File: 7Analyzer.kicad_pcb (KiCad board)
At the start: 2 copper layers, 51.3 x 72.1 mm, 30 parts, among them J1 PINHD_1x1_Male, J10 PINHD_1x3_Male, J11 PINHD_1x3_Male, J2 PINHD_1x1_Male, J3 PINHD_1x3_Male, J4 PINHD_1x3_Male, J5 PINHD_1x3_Male, J6 PINHD_1x3_Male, J7 PINHD_1x3_Male, J8 PINHD_1x3_Male, J9 PINHD_1x3_Male, P1 USB_C_Plug, U1 ESP32-DevKitC

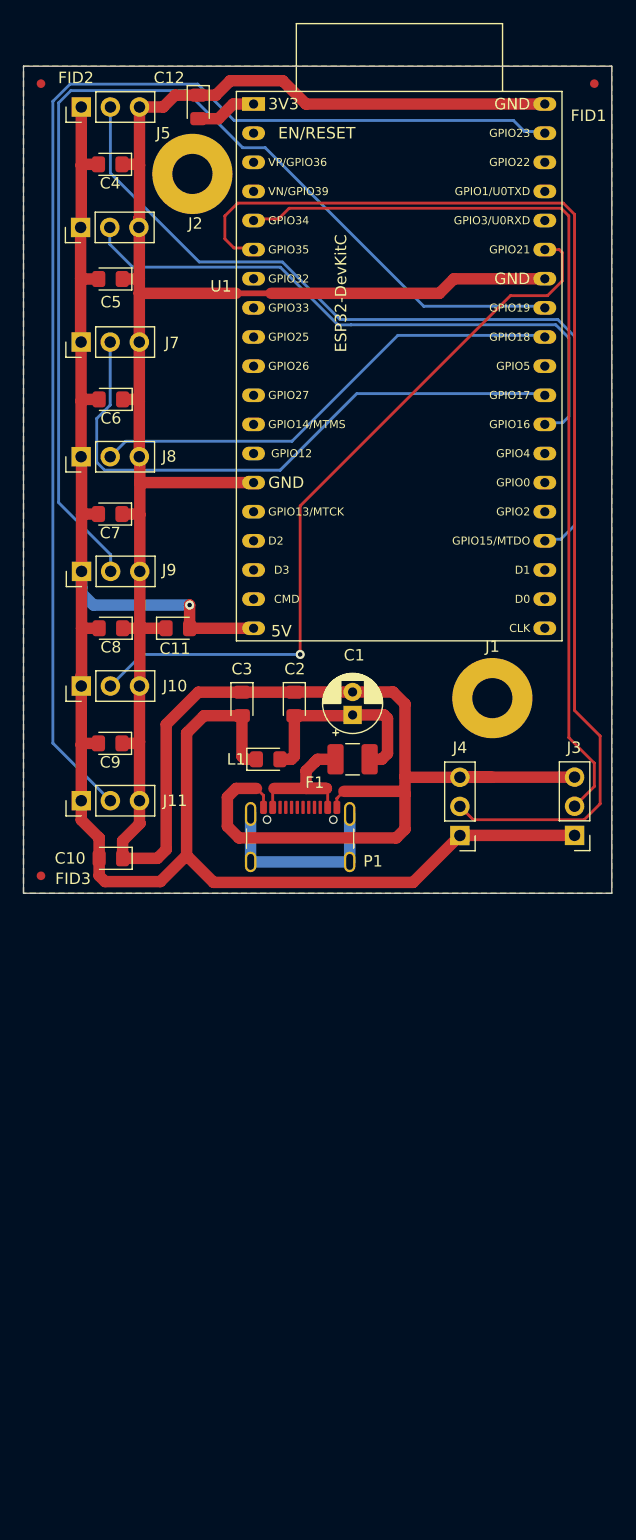
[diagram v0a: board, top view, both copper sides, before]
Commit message: laengere Version
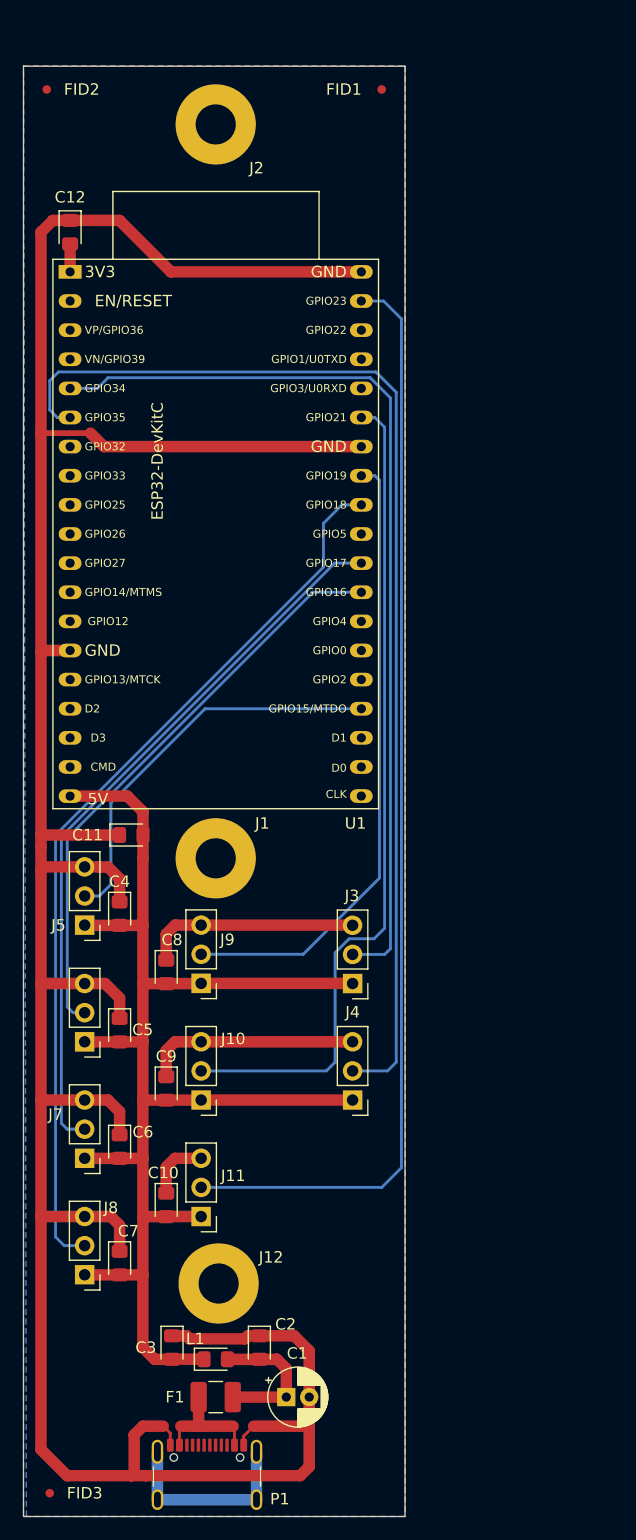
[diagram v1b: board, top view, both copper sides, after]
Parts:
- added J12: PINHD_1x1_Male, MountingHole:MountingHole_3.5mm_Pad, F.Cu at (29.0, 118.1)
- moved J5 71.4 mm to (17.3, 86.9), turned to 180 degrees
- moved J8 71.3 mm to (17.3, 117.3), turned to 180 degrees
- moved J7 71.2 mm to (17.3, 107.2), turned to 180 degrees
- moved J6 71.0 mm to (17.3, 97.0), turned to 180 degrees
- moved C5 65.5 mm to (20.3, 96.0), turned to -90 degrees
- moved C4 65.4 mm to (20.3, 85.9), turned to -90 degrees
- moved C7 65.3 mm to (20.3, 116.3), turned to -90 degrees
- moved C6 65.2 mm to (20.3, 106.2), turned to -90 degrees
- moved C1 59.8 mm to (34.9, 128.0), turned to 0 degrees
- moved F1 56.9 mm to (28.7, 128.0)
- moved C3 56.5 mm to (24.9, 123.7)
- moved C2 56.2 mm to (32.5, 123.7)
- moved P1 56.2 mm to (27.9, 135.9)
- moved FID3 53.9 mm to (14.2, 136.4)
- moved L1 52.5 mm to (28.7, 124.7)
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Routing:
- net GND: track 257.4 -> 317.8 mm
- net +5V: track 162.9 -> 121.5 mm, vias 1 -> 0
- net /A19: track 93.2 -> 54.7 mm
- net /A15: track 71.9 -> 35.1 mm
- net /A18: track 42.1 -> 78.7 mm
- net /A23: track 108.1 -> 96.4 mm
- net /A17: track 52.9 -> 63.3 mm
- net /A21: track 65.7 -> 72.8 mm, vias 1 -> 0
- net Net-(L1--): track 17.5 -> 12.6 mm
- net Net-(F1-Pad1): track 14.3 -> 10.5 mm
- net /A16: track 54.3 -> 51.0 mm
- net /A35: track 101.6 -> 98.4 mm
- net +3.3V: track 5.36 -> 2.44 mm
- net /A34: track 81.5 -> 80.6 mm
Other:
- board size 51.3 x 72.1 mm -> 33.3 x 126.5 mm
